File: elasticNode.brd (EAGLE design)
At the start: 58.2 x 52.5 mm, 115 parts, among them J1 FEMALE_HEADER_2X1, J2 JUMPER, J3 ISP_CONN_6PIN, J5 FEMALE_HEADER_10X2, J6 USB_CONNMICRO_SMT, M1 SISS23DN, M2 SISS23DN, M3 SISS23DN, U1 AT90USB128, U10 LTC3419DFN, U11 PAC1720, U12 MT41J128M8, U14 LTC3419DFN, U3 MRF24J40MA, U4 SPARTAN7-LX15, U6 SST26VF032BWDFN, U7 PAC1720, U8 PAC1720, U9 PAC1720, X1 8MHz, X2 50MHz, X3 32MHz, X4 100MHz

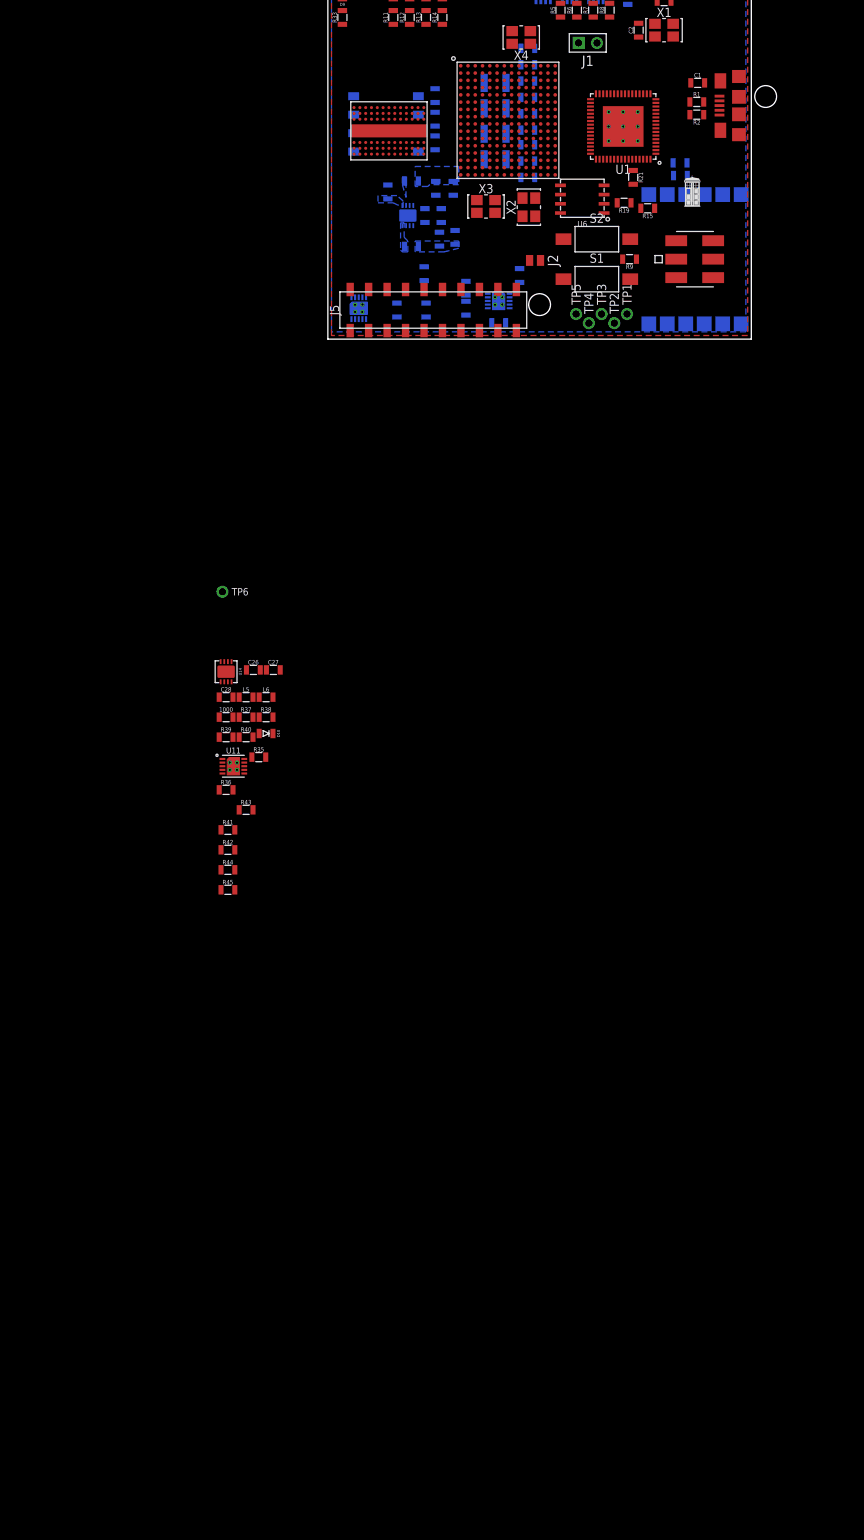
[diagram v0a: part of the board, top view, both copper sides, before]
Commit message: backup before review
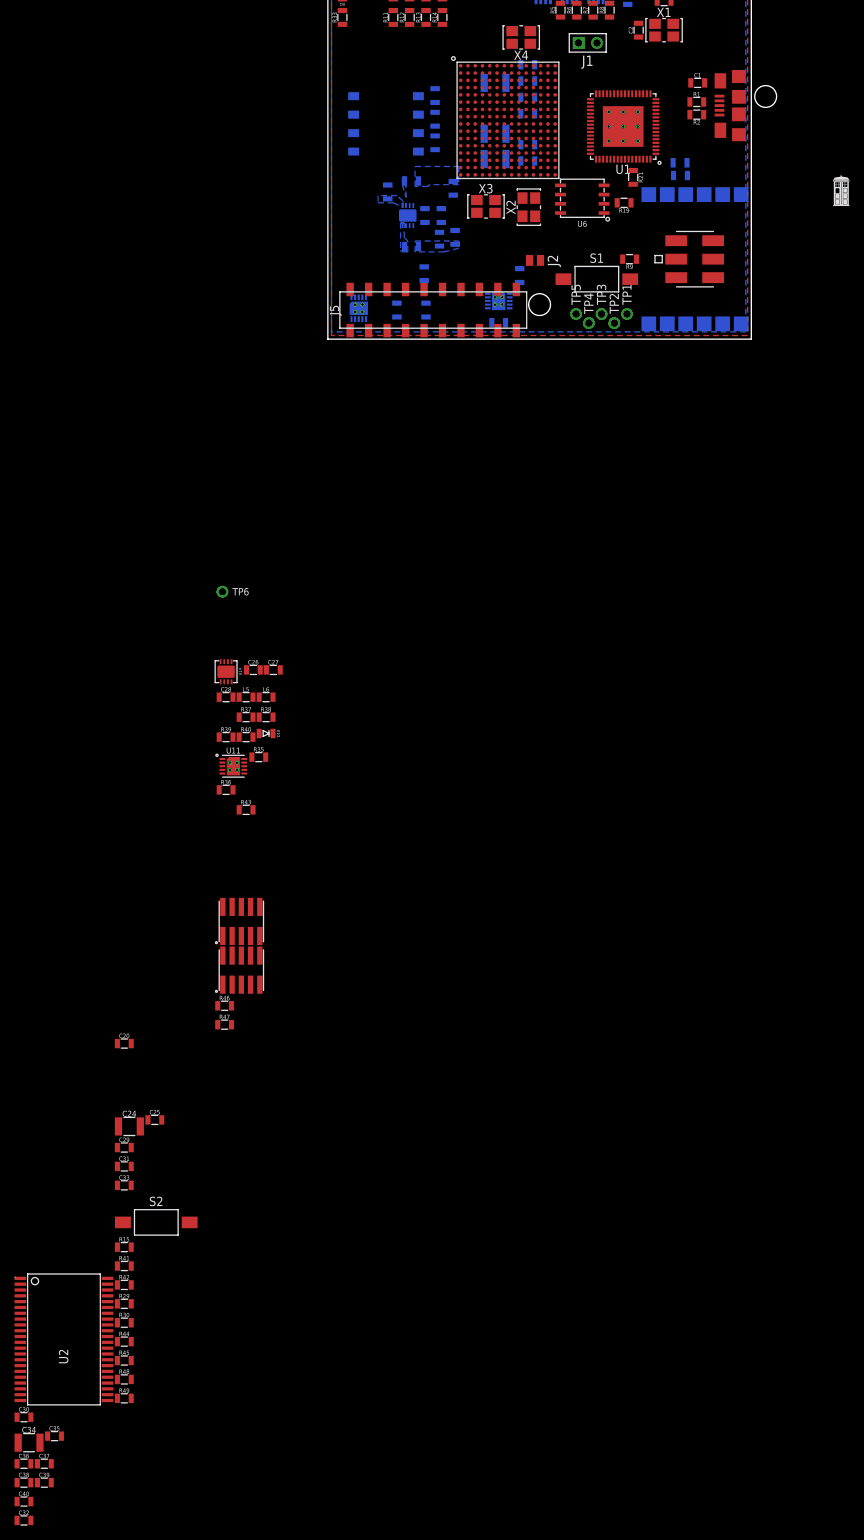
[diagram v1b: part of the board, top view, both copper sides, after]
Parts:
- removed 1000: 6k8, passive:0805
- removed 2.2K: 1k5, passive:0805
- removed C12, C9: 10u, passive:0805
- removed C15: 4.7u, passive:0805
- removed C6: 100u, passive:1210
- removed U12: MT41J128M8, ic:FBGA78DA
- added C20, C31, C32, C33, C37, C38, C39: 0.47u, passive:0805
- added C24, C34: 100u, passive:1210
- added C25, C29, C30, C35, C36, C40: 4.7u, passive:0805
- added OUT1, OUT2: FEMALE_HEADER_5X2, connectors:5X2_HEADER_SMT_1.27
- added R46: 10k, passive:0805
- added R47: 20k, passive:0805
- added R48, R49: 1.5k, passive:0805
- added U2: IS66WV51216EALL, ic:TSOP44
- C1: value (none) -> 10u
- C13: value 10u -> 0.47u
- C16: value 2.2u -> 0.47u
- C7: value 47u -> 4.7u
- R34: value 1k5 -> 10k
- R39: value 1k5 -> 6k8
- R41, R42: value 10k -> 1.5k
- R44: value 240%1 -> 1.5k
- R45: value 80.6 -> 1.5k
- moved R15 160.0 mm to (-28.0, -124.9), turned to 0 degrees
- moved S2 148.2 mm to (-23.6, -121.5)
- moved R29 147.4 mm to (-28.0, -132.7), flipped to the top, turned to 0 degrees
- moved R30 147.3 mm to (-28.0, -135.3), flipped to the top, turned to 0 degrees
- moved R44 66.4 mm to (-28.0, -137.9)
- moved R45 66.3 mm to (-28.0, -140.5)
- moved R41 61.7 mm to (-28.0, -127.5)
- moved R42 61.5 mm to (-28.0, -130.1)
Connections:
- removed net DDR_A0: U12.K3, U4.B3
- removed net DDR_A1: U12.L7, U4.N1
- removed net DDR_A10: U12.H7, U4.M2
- removed net DDR_A11: U12.M7, U4.P2
- removed net DDR_A12: U12.K7, U4.M4
- removed net DDR_A13: U12.N3, U4.A5
- removed net DDR_A2: U12.L3, U4.B6
- removed net DDR_A3: U12.K2, U4.B2, U4.F4
- removed net DDR_A4: U12.L8, U4.M5
- removed net DDR_A5: U12.L2, U4.B5
- removed net DDR_A6: U12.M8, U4.N4
- removed net DDR_A7: U12.M2, U4.A2
- removed net DDR_A8: U12.N8, U4.P5
- removed net DDR_A9: U12.M3, U4.A3
- removed net DDR_BA0: U12.J2, U4.C5
- removed net DDR_BA1: U12.K8, U4.M3
- removed net DDR_BA2: U12.J3, U4.B1
- removed net DDR_CAS: U12.G3, U4.C1
- removed net DDR_CKE: U12.G9, U4.M1
- removed net DDR_CLK_N: R45.1, U12.G7, U4.P3
- removed net DDR_CLK_P: R45.2, U12.F7, U4.P4
- removed net DDR_CS: U12.H2, U4.C3
- removed net DDR_DQ0: U12.B3, U4.E2
- removed net DDR_DQ1: U12.C7, U4.L2
- removed net DDR_DQ2: U12.C2, U4.E4
- removed net DDR_DQ3: U12.C8, U4.L1
- removed net DDR_DQ4: U12.E3, U4.D2
- removed net DDR_DQ5: U12.E8, U4.L3
- removed net DDR_DQ6: U12.D2, U4.D1
- removed net DDR_DQ7: U12.E7, U4.L5
- removed net DDR_DQS_N: U12.D3, U4.F1
- removed net DDR_DQS_P: U12.C3, U4.G1
- removed net DDR_ODT: U12.G1, U4.D4
- removed net DDR_RAS: U12.F3, U4.D3
- removed net DDR_RESET: U12.N2, U4.A4
- removed net DDR_WE: U12.H3, U4.C4
- removed net N$18: U4.B10
- removed net N$37: U4.H14
- removed net N$38: U4.H13
- removed net N$43: U4.F3
- removed net N$44: U4.F2
- removed net N$52: U4.H4
- removed net N$58: U4.C12
- removed net N$59: U4.H3
- removed net N$60: U4.H2
- removed net N$61: U4.H1
- removed net N$62: U4.J2
- removed net N$63: U4.J1
- removed net N$64: U4.K4
- removed net N$65: U4.K3
- removed net N$66: U4.J4
- removed net N$67: U4.J3
- removed net N$69: R44.1, U12.H8
- removed net VCC_DDR: R23.2, R41.2, R43.2, U11.2, U12.A2, U12.A9, U12.B9, U12.C1, U12.D7, U12.E2, U12.E9, U12.G2, U12.G8, U12.K1, U12.K9, U12.M1, U12.M9, U4.G2, U4.K2, U4.N2, U7.2, X4.1, X4.4
- removed net VREF_DDR: R41.1, R42.2, U12.E1, U12.J8
- new net 1V8: C19.2, L2.2, R23.1, R25.2, R43.1, R47.2, TP2.3, U11.1, U7.1, U9.1
- new net N$21: U4.P4
- new net N$22: U4.P3
- new net N$26: U4.L3
- new net N$31: U4.L2
- new net N$33: U4.M5
- new net N$34: U4.M4
- new net N$35: U4.P5
- new net N$36: U4.N4
- new net N$40: U4.L5
- new net SRAM_A0: U2.5, U4.D3
- new net SRAM_A1: U2.4, U4.C3
- new net SRAM_A10: U2.25, U4.C5
- new net SRAM_A11: U2.24, U4.C4
- new net SRAM_A12: U2.22, U4.E4
- new net SRAM_A13: U2.21, U4.D4
- new net SRAM_A14: U2.20, U4.F3
- new net SRAM_A15: U2.19, U4.F2
- new net SRAM_A16: U2.18, U4.G1
- new net SRAM_A17: U2.23, U4.F1
- new net SRAM_A18: U2.28, U4.E2
- new net SRAM_A2: U2.3, U4.A4
- new net SRAM_A3: U2.2, U4.A3
- new net SRAM_A4: U2.1, U4.B3
- new net SRAM_A5: U2.44, U4.A2
- new net SRAM_A6: U2.43, U4.B5
- new net SRAM_A7: U2.42, U4.A5
- new net SRAM_A8: U2.27, U4.B2
- new net SRAM_A9: U2.26, U4.B1
- new net SRAM_CS: U2.6, U4.B6
- new net SRAM_D0: U2.7, U4.D2
- new net SRAM_D1: U2.8, U4.D1
- new net SRAM_D10: U2.31, U4.K3
- new net SRAM_D11: U2.32, U4.J4
- new net SRAM_D12: U2.35, U4.J3
- new net SRAM_D13: U2.36, U4.M1
- new net SRAM_D14: U2.37, U4.L1
- new net SRAM_D15: U2.38, U4.M3
- new net SRAM_D2: U2.9, U4.C1
- new net SRAM_D3: U2.10, U4.H4
- new net SRAM_D4: U2.13, U4.H3
- new net SRAM_D5: U2.14, U4.H2
- new net SRAM_D6: U2.15, U4.H1
- new net SRAM_D7: U2.16, U4.J2
- new net SRAM_D8: U2.29, U4.J1
- new net SRAM_D9: U2.30, U4.K4
- new net SRAM_LB: U2.39, U4.N1
- new net SRAM_OE: U2.41, U4.M2
- new net SRAM_UB: U2.40, U4.P2
- new net SRAM_VCC: R23.2, R43.2, U11.2, U4.G2, U4.K2, U4.N2, U7.2, X4.1, X4.4
- new net SRAM_VDD: C24.1, C25.1, C29.1, C30.1, C31.1, C32.1, C33.1, U2.11, U2.33
- new net SRAM_WE: U2.17, U4.F4
- net 1V: now also R46.2; no longer 1000.1
- net 1V2: no longer R25.2, U9.1
- net 1V5: no longer 2.2K.2, C19.2, L2.2, R23.1, R43.1, U11.1, U7.1
- net 3V3: now also OUT2.10, R30.2, R41.2, R42.2, R44.2, R45.2, R48.2, R49.2; no longer R30.1, TP2.3
- net 5V: now also OUT2.9, R36.2, U11.3; no longer R36.1, U11.4
- net A10: now also OUT1.5
- net A11: now also OUT1.6
- net A12: now also OUT1.7
- net A13: now also OUT1.8
- net A14: now also OUT1.10
- net A8: now also OUT1.3
- net A9: now also OUT1.4
- net AD0/SELECTMAP_D7: now also OUT2.1
- net AD1/SELECTMAP_D6: now also OUT2.2
- net AD2/SELECTMAP_D5/MCU_RX1: now also OUT2.3
- net AD3/SELECTMAP_D4/MCU_TX1: now also OUT2.4
- net AD4/SELECTMAP_D3/FPGA_HOLD: now also OUT2.5
- net AD5/SELECTMAP_D2/FPGA_WP: now also OUT2.6
- net ALE/HWB: now also OUT1.9
- net FPGA_GPIO_18: now also U4.H14
- net FPGA_GPIO_19: now also U4.H13
- net FPGA_LED0: now also U4.E11
- net FPGA_LED1: now also U4.B10
- net FPGA_LED2: now also U4.A10
- net FPGA_LED3: now also U4.C12
- net FPGA_VCCAUX: now also C20.1
- net FPGA_VCCIO: now also C34.1, C35.1, C36.1, C37.1, C38.1, C39.1, C40.1; no longer C12.1, C15.1, C6.1, C9.1, R20.1, U7.4
- net FPGA_VCCIO_MON: now also R20.1, U7.4
- net GND: now also C20.2, C24.2, C25.2, C29.2, C30.2, C31.2, C32.2, C33.2, C34.2, C35.2, C36.2, C37.2, C38.2, C39.2, C40.2, OUT2.7, OUT2.8, U2.12, U2.34; no longer C12.2, C15.2, C6.2, C9.2, R42.1, R44.2, U12.A1, U12.A8, U12.B1, U12.B2, U12.B7, U12.B8, U12.C9, U12.D1, U12.D8, U12.D9, U12.F2, U12.F8, U12.J1, U12.J9, U12.L1, U12.L9, U12.N1, U12.N9
- net N$53: now also R46.1; no longer 1000.2
- net N$7: now also R47.1; no longer 2.2K.1
- net SCL: now also OUT1.1, R41.1, R44.1, R48.1
- net SDA: now also OUT1.2, R30.1, R42.1, R45.1, R49.1; no longer R30.2
- net USB_VCC_RAW: now also R36.1, U11.4; no longer R36.2, U11.3

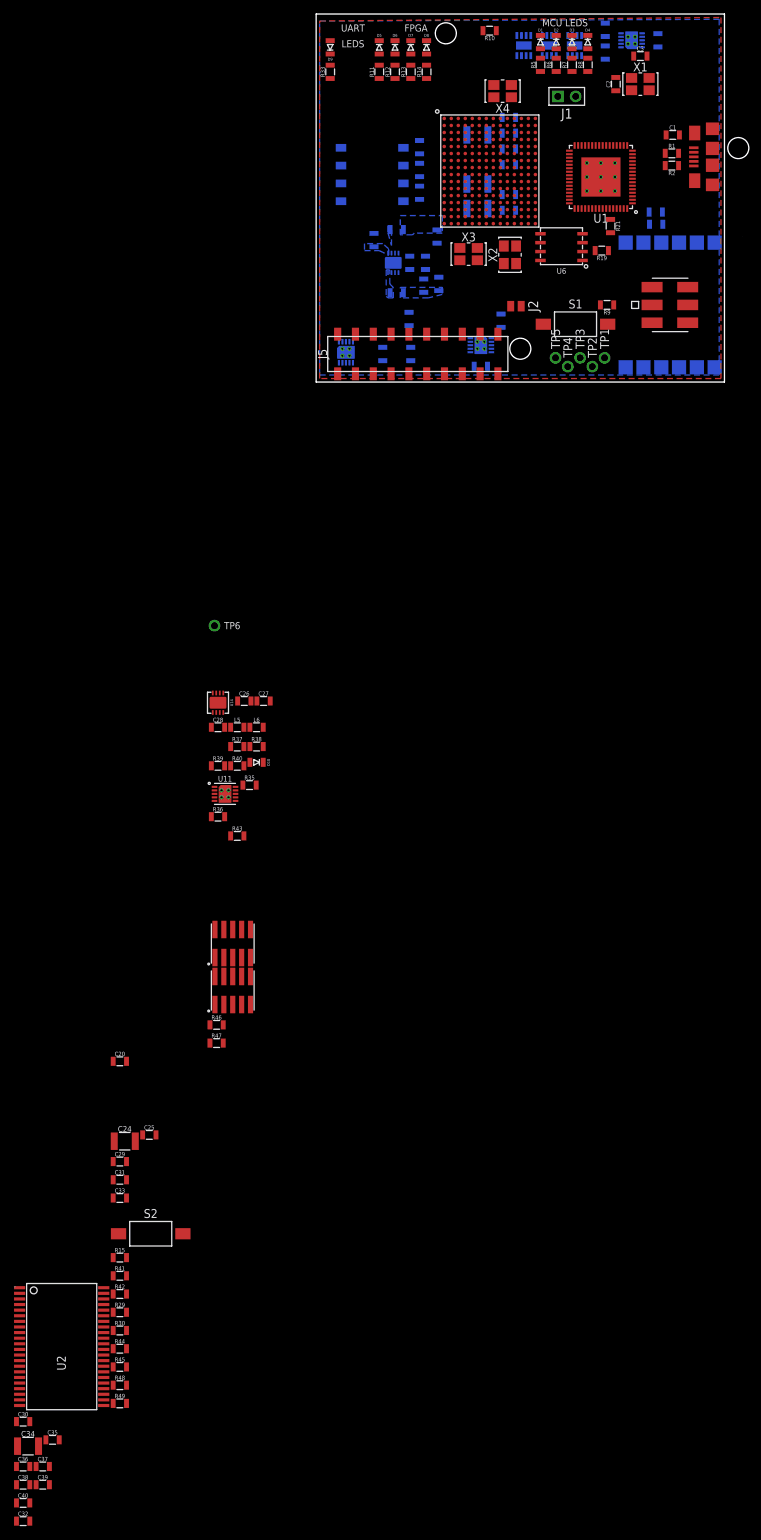
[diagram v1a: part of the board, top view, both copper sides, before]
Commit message: back up before review.
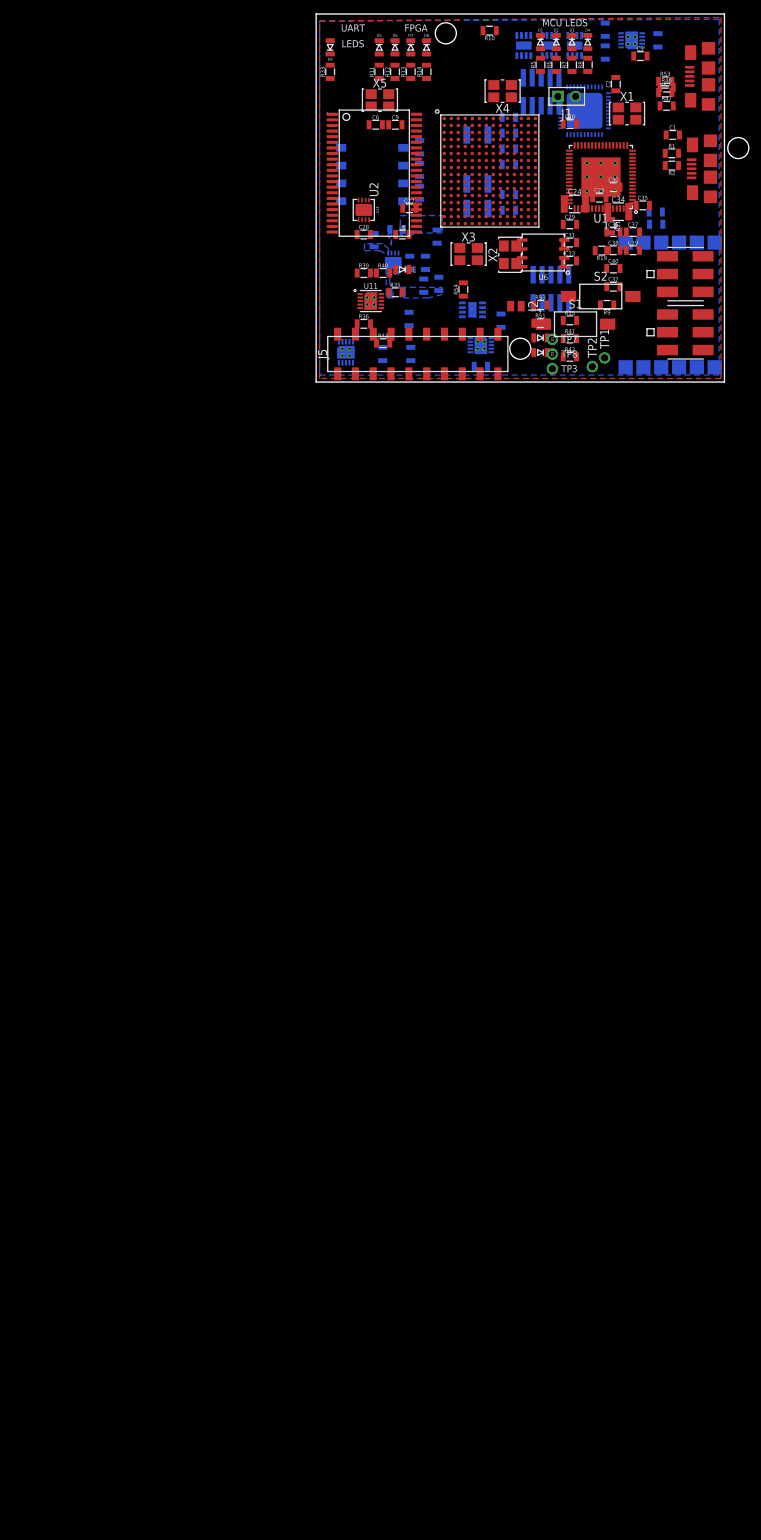
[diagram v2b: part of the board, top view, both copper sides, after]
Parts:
- removed C26: 22u, passive:0805
- removed J3: ISP_CONN_6PIN, connectors:ICSP_SMT
- removed L5: 3.3uH, passive:0805
- removed R29, R30, R44, R45, R48, R49: 1.5k, passive:0805
- removed R37, R38: 1k5, passive:0805
- removed TP4, TP5, TP6: TEST_POINTTHT, connectors:THT
- added C6, C9: 20p, passive:0805
- added D11, D12: GREEN 2.2V, opto:0805
- added J7: USB_CONNMICRO_SMT, connectors:USB_MICRO_B_SMT
- added M4: SISS23DN, power:POWERPAK1212-8
- added MCU_PROGRAM, MON_PROGRAM: ISP_CONN_6PIN, connectors:ICSP_SMT
- added R50, R51: 550, passive:0805
- added R52, R53: 22, passive:0805
- added R54: 15k, passive:0805
- added TP7, TP8: TEST_POINTTHT, connectors:THT
- added U5: ATMEGA32U4QFN, ic:QFN44
- added X5: 8MHz, passive:3.2X2.5_OSC
- moved C30 195.2 mm to (42.4, 27.8)
- moved C34 195.2 mm to (43.1, 24.3)
- moved C38 195.2 mm to (42.4, 18.8)
- moved C39 195.2 mm to (45.2, 18.8)
- moved C32 195.2 mm to (42.4, 13.6)
- moved C35 195.2 mm to (46.6, 25.2)
- moved C36 195.2 mm to (42.4, 21.4)
- moved C37 195.2 mm to (45.2, 21.4)
- moved C40 195.2 mm to (42.4, 16.2)
- moved U2 173.2 mm to (8.30, 29.8)
- moved C20 148.3 mm to (36.2, 36.8)
- moved C24 148.3 mm to (36.9, 25.4)
- moved C25 148.3 mm to (40.4, 26.3)
- moved C29 148.3 mm to (36.2, 22.5)
- moved C31 148.3 mm to (36.2, 19.9)
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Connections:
- net A10 renamed XMEM_A10
- net A11 renamed XMEM_A11
- net A12 renamed XMEM_A12
- net A13 renamed XMEM_A13
- net A14 renamed XMEM_A14
- net A15 renamed XMEM_A15
- net A8 renamed XMEM_A8
- net A9 renamed XMEM_A9
- net RD renamed XMEM_RD
- net WR renamed XMEM_WR
- removed net 1V2: C26.2, L5.2, R37.2, TP3.3
- removed net 1V5: TP6.3
- removed net ENABLE_LEDS: U1.17
- removed net FPGA_RESES: U1.59
- removed net FPGA_SUSPEND: U1.19
- removed net N$21: U4.P4
- removed net N$22: U4.P3
- removed net N$26: U4.L3
- removed net N$31: U4.L2
- removed net N$33: U4.M5
- removed net N$34: U4.M4
- removed net N$35: U4.P5
- removed net N$36: U4.N4
- removed net N$39: U4.H12
- removed net N$40: U4.L5
- removed net N$54: R37.1, R38.2, U14.8
- removed net N$56: L5.1, U14.6
- removed net SRAM_VCC: R23.2, R43.2, U11.2, U4.G2, U4.K2, U4.N2, U7.2, X4.1, X4.4
- new net DAUGHTER_VCC: OUT2.10, R43.2, U11.2
- new net GND1: D11.2, D12.2
- new net MON_LED0: R50.1, U5.20
- new net MON_LED1: R51.1, U5.21
- new net MON_MISO: MON_PROGRAM.1, U5.11
- new net MON_MOSI: MON_PROGRAM.4, U5.10
- new net MON_RESET: MON_PROGRAM.5, R54.2, U5.13
- new net MON_SCK: MON_PROGRAM.3, U5.9
- new net MON_USB_D+: R53.1, U5.4
- new net MON_USB_D-: R52.1, U5.3
- new net MON_USB_VCC: J7.1, U5.7
- new net N$16: D12.1, R51.2
- new net N$17: D11.1, R50.2
- new net N$18: C9.1, U5.17, X5.3
- new net N$19: J7.2, R52.2
- new net N$20: C6.1, U5.16, X5.1
- new net SRAM_POWER: M4.4, U1.2
- new net SRAM_VDD_MON: M4.1, M4.2, M4.3, R23.2, U7.2
- net 1V: now also TP8.3; no longer TP4.3
- net 1V8: now also TP7.3; no longer R43.1, TP2.3, U11.1
- net 3V3: now also MCU_PROGRAM.2, MON_PROGRAM.2, R43.1, R54.1, TP2.3, U11.1, U5.14, U5.2, U5.24, U5.34, U5.44, U5.6; no longer J3.2, OUT2.10, R29.2, R30.2, R44.2, R45.2, R48.2, R49.2, U14.7
- net AD6/SELECTMAP_D1/SPI_MISO/MCU_PDO: now also MCU_PROGRAM.1; no longer J3.1
- net AD7/SELECTMAP_D0/SPI_MOSI/PDI: now also MCU_PROGRAM.4; no longer J3.4
- net FPGA_RESET: now also U1.59
- net GND: now also C2.2, C3.2, C6.2, C9.2, J7.5, MCU_PROGRAM.6, MON_PROGRAM.6, TP3.3, U5.15, U5.23, U5.35, U5.43, U5.45, U5.5; no longer C26.1, J3.6, R38.1, TP5.3
- net MCU_RESET: now also MCU_PROGRAM.5; no longer J3.5
- net MONITORING: now also U5.1
- net N$5: now also J7.3, R53.2; no longer C2.2, C3.2
- net SCL: now also U5.18; no longer R29.1, R44.1, R48.1
- net SDA: now also U5.19; no longer R30.1, R45.1, R49.1
- net SPI_SCK/CCLK: now also MCU_PROGRAM.3; no longer J3.3
- net SRAM_VDD: now also M4.5, M4.6, M4.7, M4.8, U4.G2, U4.K2, U4.N2, X4.1, X4.4

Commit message: Layout work start.
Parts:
- removed C18: 10u, passive:0805
- removed D10: RED, opto:0805
- removed R39: 6k8, passive:0805
- removed R40: 270, passive:0805
- removed R46: 10k, passive:0805
- added C12, C15: 10u, passive:0805
- added J3: JUMPER, connectors:JUMPER_SMT
- added R29, R30: 15k, passive:0805
- added R37: 1k5, passive:0805
- added R38: 6k8, passive:0805
- R31: value 6k8 -> 10k
- R32: value 1k5 -> 6k8
- moved R1 157.5 mm to (204.6, 66.6)
- moved R2 157.5 mm to (204.6, 64.9)
- moved U7 117.0 mm to (93.3, 80.1), flipped to the top, turned to 0 degrees
- moved R26 111.2 mm to (93.4, 77.0), flipped to the top, turned to 0 degrees
- moved D9 107.1 mm to (-20.8, -56.9), turned to 0 degrees
- moved R20 107.0 mm to (89.9, 78.9), flipped to the top
- moved R23 105.8 mm to (89.9, 81.9), flipped to the top
- moved R33 101.6 mm to (-20.8, -54.8), turned to 0 degrees
- moved U11 98.5 mm to (93.3, 60.4)
- moved R43 98.3 mm to (89.9, 62.2), turned to 90 degrees
- moved U8 97.6 mm to (93.3, 73.4), flipped to the top
- moved R27 97.6 mm to (93.4, 70.3), flipped to the top
- moved R36 97.4 mm to (89.9, 59.2), turned to 90 degrees
- moved R42 97.2 mm to (19.5, 99.4)
- moved R41 95.2 mm to (16.7, 99.4)
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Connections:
- removed net N$1: L1.2, U10.4
- removed net N$57: D10.2, R40.2
- removed net N$8: L2.1, U10.6
- new net MON_HWB: J3.1, R30.2, U5.33
- new net N$21: R29.1, U5.2
- new net N$22: L1.1, U10.4
- new net N$26: L2.2, U10.6
- net 1V: now also C17.1, L1.2, R31.2; no longer C27.1, L6.1, R46.2
- net 1V8: now also L2.1, R23.2, R47.1; no longer L2.2, R23.1, R47.2
- net 3V3: now also C12.1, C27.1, L6.1, R24.2, R29.2, R30.1, R38.2, R43.2; no longer C17.1, L1.1, R24.1, R31.1, R43.1, U5.2
- net 5V: now also C15.1; no longer C18.1, D10.1, D9.1
- net DAUGHTER_VCC: now also R43.1; no longer R43.2
- net GND: now also C12.2, C15.2, J3.2, R37.2; no longer C18.2, R39.2, R40.1
- net MONITORING: now also U1.1
- net N$2: now also R31.1; no longer R31.2
- net N$53: now also R37.1, R38.1; no longer R39.1, R46.1
- net N$7: now also R47.2; no longer R47.1
- net SRAM_VDD_MON: now also R23.1; no longer R23.2
- net USB_VCC_RAW: now also D9.1
- net WIRELESS_VCC: now also R24.1; no longer R24.2
